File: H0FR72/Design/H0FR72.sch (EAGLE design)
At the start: 49 parts, among them P1 HEXABIT_17.32_NO_P6_P7_P12, Q1 MMBT3904LT1, Q2 STD36P4LLF6, U1 STM32G0B1CEU6N, U2 TSV772IYDT, U3 PMD3001D,115, X1 XTALL_CSTCE8M00G52

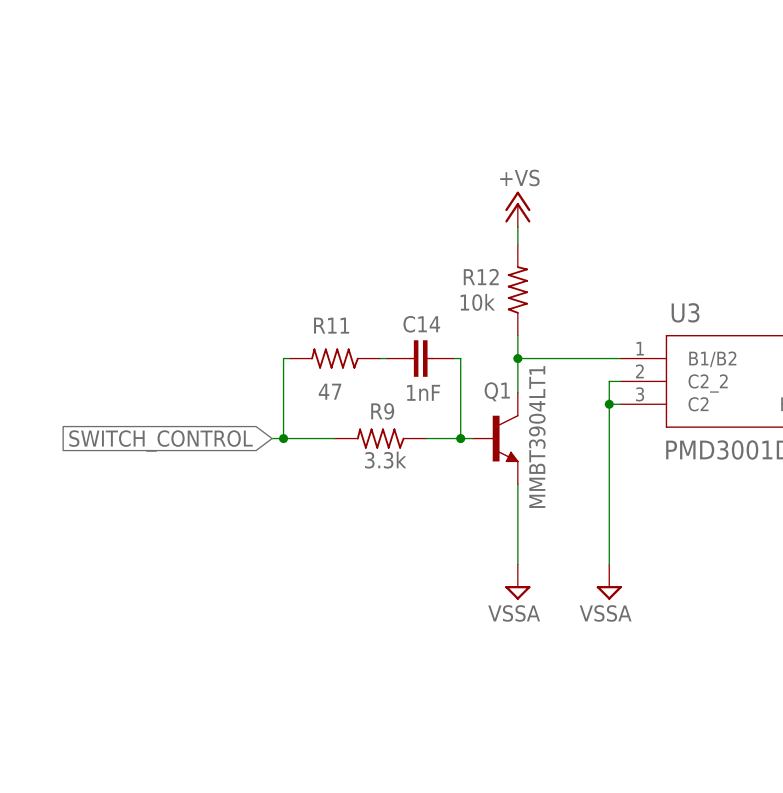
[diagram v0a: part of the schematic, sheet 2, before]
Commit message: Schematic modification
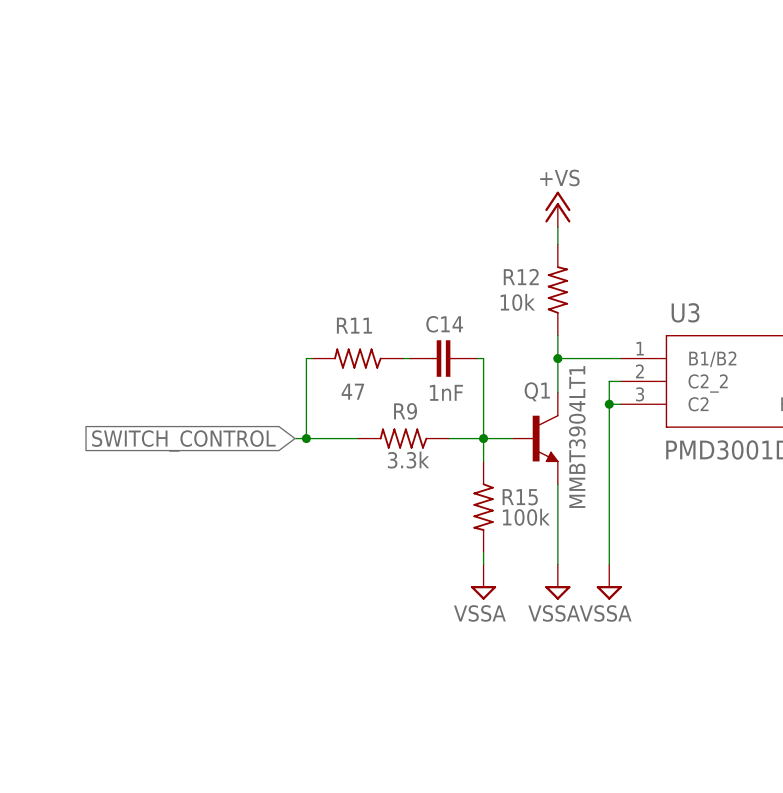
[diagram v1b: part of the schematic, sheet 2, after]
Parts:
- added R15: 100k, HEXABITZ_RCLS:R-0402
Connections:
- net N$14: now also R15.1
- net VSSA: now also R15.2
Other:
- moved on the sheet: C14, Q1, R11, R12, R9
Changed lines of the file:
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@@
 <part name="SUPPLY18" library="supply2" deviceset="VDD" device=""/>
 <part name="SUPPLY19" library="HEXABITZ_CONNECTION_PARTS" library_urn="urn:adsk.eagle:library:20064553" deviceset="VSSA" device=""/>
+<part name="R15" library="HEXABITZ_RCLS" library_urn="urn:adsk.eagle:library:20064561" deviceset="R-0402" device="" package3d_urn="urn:adsk.eagle:package:19666455/3" value="100k">
+<attribute name="MFN" value="Yageo"/>
+<attribute name="MPN" value="RC0603JR-07680KL"/>
+<attribute name="OCTOPART_URL" value="https://octopart.com/rc0603jr-07680kl-yageo-40953169?r=sp"/>
+<attribute name="RESISTANCE" value="680K Ohm"/>
+<attribute name="TOLERANCE" value="5%"/>
+</part>
+<part name="SUPPLY21" library="HEXABITZ_CONNECTION_PARTS" library_urn="urn:adsk.eagle:library:20064553" deviceset="VSSA" device=""/>
 </parts>
 <sheets>
@@
 <attribute name="VALUE" x="249.555" y="85.09" size="1.778" layer="96" rot="R180"/>
 </instance>
-<instance part="R12" gate="G$1" x="64.77" y="135.89" smashed="yes" rot="R90">
-<attribute name="NAME" x="62.865" y="138.2014" size="1.778" layer="95" rot="R180"/>
-<attribute name="VALUE" x="62.23" y="135.382" size="1.778" layer="96" rot="R180"/>
+<instance part="R12" gate="G$1" x="69.215" y="135.89" smashed="yes" rot="R90">
+<attribute name="NAME" x="67.31" y="138.2014" size="1.778" layer="95" rot="R180"/>
+<attribute name="VALUE" x="66.675" y="135.382" size="1.778" layer="96" rot="R180"/>
 </instance>
 <instance part="R5" gate="G$1" x="120.65" y="127.635" smashed="yes" rot="R180">
@@
 <attribute name="POWER" x="124.46" y="126.365" size="1.778" layer="96" rot="R180"/>
 </instance>
-<instance part="Q1" gate="G$1" x="62.23" y="119.38" smashed="yes">
-<attribute name="NAME" x="60.96" y="123.825" size="1.778" layer="95"/>
-<attribute name="VALUE" x="66.04" y="127.635" size="1.778" layer="96" rot="R270"/>
+<instance part="Q1" gate="G$1" x="66.675" y="119.38" smashed="yes">
+<attribute name="NAME" x="65.405" y="123.825" size="1.778" layer="95"/>
+<attribute name="VALUE" x="70.485" y="127.635" size="1.778" layer="96" rot="R270"/>
 </instance>
 <instance part="U3" gate="A" x="91.44" y="125.73" smashed="yes">
@@
 <attribute name="VALUE" x="116.84" y="140.843" size="1.778" layer="96"/>
 </instance>
-<instance part="R9" gate="G$1" x="49.53" y="119.38" smashed="yes" rot="R180">
-<attribute name="NAME" x="48.26" y="121.5136" size="1.778" layer="95"/>
-<attribute name="VALUE" x="47.625" y="116.078" size="1.778" layer="96"/>
-</instance>
-<instance part="C14" gate="G$1" x="55.245" y="128.27" smashed="yes" rot="R90">
-<attribute name="NAME" x="56.261" y="132.969" size="1.778" layer="95" rot="R180"/>
-<attribute name="VALUE" x="56.261" y="125.349" size="1.778" layer="96" rot="R180"/>
-</instance>
-<instance part="R11" gate="G$1" x="44.45" y="128.27" smashed="yes" rot="R180">
-<attribute name="NAME" x="41.91" y="131.0386" size="1.778" layer="95"/>
-<attribute name="VALUE" x="42.545" y="123.698" size="1.778" layer="96"/>
+<instance part="R9" gate="G$1" x="52.07" y="119.38" smashed="yes" rot="R180">
+<attribute name="NAME" x="50.8" y="121.5136" size="1.778" layer="95"/>
+<attribute name="VALUE" x="50.165" y="116.078" size="1.778" layer="96"/>
+</instance>
+<instance part="C14" gate="G$1" x="57.785" y="128.27" smashed="yes" rot="R90">
+<attribute name="NAME" x="58.801" y="132.969" size="1.778" layer="95" rot="R180"/>
+<attribute name="VALUE" x="58.801" y="125.349" size="1.778" layer="96" rot="R180"/>
+</instance>
+<instance part="R11" gate="G$1" x="46.99" y="128.27" smashed="yes" rot="R180">
+<attribute name="NAME" x="44.45" y="131.0386" size="1.778" layer="95"/>
+<attribute name="VALUE" x="45.085" y="123.698" size="1.778" layer="96"/>
 </instance>
 <instance part="P+1" gate="1" x="15.875" y="198.755" smashed="yes">
@@
 <attribute name="VALUE" x="161.925" y="187.96" size="1.778" layer="96" rot="R180"/>
 </instance>
-<instance part="SUPPLY12" gate="G$1" x="64.77" y="102.87" smashed="yes">
-<attribute name="VALUE" x="61.468" y="99.06" size="1.778" layer="96"/>
+<instance part="SUPPLY12" gate="G$1" x="69.215" y="102.87" smashed="yes">
+<attribute name="VALUE" x="65.913" y="99.06" size="1.778" layer="96"/>
 </instance>
 <instance part="C15" gate="G$1" x="167.64" y="179.705" smashed="yes" rot="R270">
@@
 <attribute name="VALUE" x="110.49" y="157.48" size="1.778" layer="96" rot="R180"/>
 </instance>
-<instance part="P+4" gate="1" x="64.77" y="145.415" smashed="yes">
-<attribute name="VALUE" x="67.31" y="149.225" size="1.778" layer="96" rot="R180"/>
+<instance part="P+4" gate="1" x="69.215" y="145.415" smashed="yes">
+<attribute name="VALUE" x="71.755" y="149.225" size="1.778" layer="96" rot="R180"/>
 </instance>
 <instance part="SUPPLY19" gate="G$1" x="167.64" y="162.56" smashed="yes">
 <attribute name="VALUE" x="164.338" y="158.75" size="1.778" layer="96"/>
 </instance>
+<instance part="R15" gate="G$1" x="60.96" y="111.76" smashed="yes" rot="R270">
+<attribute name="NAME" x="62.865" y="111.9886" size="1.778" layer="95"/>
+<attribute name="VALUE" x="62.865" y="109.728" size="1.778" layer="96"/>
+</instance>
+<instance part="SUPPLY21" gate="G$1" x="60.96" y="102.87" smashed="yes">
+<attribute name="VALUE" x="57.658" y="99.06" size="1.778" layer="96"/>
+</instance>
 </instances>
 <busses>
@@
 <segment>
 <pinref part="R9" gate="G$1" pin="1"/>
-<wire x1="54.61" y1="119.38" x2="58.42" y2="119.38" width="0.1524" layer="91"/>
+<wire x1="57.15" y1="119.38" x2="60.96" y2="119.38" width="0.1524" layer="91"/>
 <pinref part="Q1" gate="G$1" pin="B"/>
-<wire x1="59.69" y1="119.38" x2="58.42" y2="119.38" width="0.1524" layer="91"/>
+<wire x1="64.135" y1="119.38" x2="60.96" y2="119.38" width="0.1524" layer="91"/>
 <pinref part="C14" gate="G$1" pin="2"/>
-<wire x1="57.785" y1="128.27" x2="58.42" y2="128.27" width="0.1524" layer="91"/>
-<wire x1="58.42" y1="128.27" x2="58.42" y2="119.38" width="0.1524" layer="91"/>
-<junction x="58.42" y="119.38"/>
+<wire x1="60.325" y1="128.27" x2="60.96" y2="128.27" width="0.1524" layer="91"/>
+<wire x1="60.96" y1="128.27" x2="60.96" y2="119.38" width="0.1524" layer="91"/>
+<junction x="60.96" y="119.38"/>
+<pinref part="R15" gate="G$1" pin="1"/>
+<wire x1="60.96" y1="116.84" x2="60.96" y2="119.38" width="0.1524" layer="91"/>
 </segment>
 </net>
@@
 <pinref part="R11" gate="G$1" pin="1"/>
 <pinref part="C14" gate="G$1" pin="1"/>
-<wire x1="49.53" y1="128.27" x2="50.165" y2="128.27" width="0.1524" layer="91"/>
+<wire x1="52.07" y1="128.27" x2="52.705" y2="128.27" width="0.1524" layer="91"/>
 </segment>
 </net>
@@
 <segment>
 <pinref part="R11" gate="G$1" pin="2"/>
-<wire x1="39.37" y1="128.27" x2="38.735" y2="128.27" width="0.1524" layer="91"/>
-<wire x1="38.735" y1="128.27" x2="38.735" y2="119.38" width="0.1524" layer="91"/>
-<label x="37.465" y="119.38" size="1.778" layer="95" rot="MR0" xref="yes"/>
+<wire x1="41.91" y1="128.27" x2="41.275" y2="128.27" width="0.1524" layer="91"/>
+<wire x1="41.275" y1="128.27" x2="41.275" y2="119.38" width="0.1524" layer="91"/>
+<label x="40.005" y="119.38" size="1.778" layer="95" rot="MR0" xref="yes"/>
 <pinref part="R9" gate="G$1" pin="2"/>
-<wire x1="38.735" y1="119.38" x2="37.465" y2="119.38" width="0.1524" layer="91"/>
-<wire x1="44.45" y1="119.38" x2="38.735" y2="119.38" width="0.1524" layer="91"/>
-<junction x="38.735" y="119.38"/>
+<wire x1="41.275" y1="119.38" x2="40.005" y2="119.38" width="0.1524" layer="91"/>
+<wire x1="46.99" y1="119.38" x2="41.275" y2="119.38" width="0.1524" layer="91"/>
+<junction x="41.275" y="119.38"/>
 </segment>
 </net>
@@
 <segment>
 <pinref part="R12" gate="G$1" pin="2"/>
-<wire x1="64.77" y1="140.97" x2="64.77" y2="142.875" width="0.1524" layer="91"/>
+<wire x1="69.215" y1="140.97" x2="69.215" y2="142.875" width="0.1524" layer="91"/>
 <pinref part="P+4" gate="1" pin="+VS"/>
 </segment>
@@
 <pinref part="Q1" gate="G$1" pin="E"/>
 <pinref part="SUPPLY12" gate="G$1" pin="VSSA"/>
-<wire x1="64.77" y1="114.3" x2="64.77" y2="105.41" width="0.1524" layer="91"/>
+<wire x1="69.215" y1="114.3" x2="69.215" y2="105.41" width="0.1524" layer="91"/>
 </segment>
 <segment>
@@
 <wire x1="167.64" y1="165.1" x2="167.64" y2="167.005" width="0.1524" layer="91"/>
 </segment>
+<segment>
+<pinref part="R15" gate="G$1" pin="2"/>
+<pinref part="SUPPLY21" gate="G$1" pin="VSSA"/>
+<wire x1="60.96" y1="106.68" x2="60.96" y2="105.41" width="0.1524" layer="91"/>
+</segment>
 </net>
 <net name="N$16" class="0">
@@
 <pinref part="Q1" gate="G$1" pin="C"/>
 <pinref part="R12" gate="G$1" pin="1"/>
-<wire x1="64.77" y1="130.81" x2="64.77" y2="128.27" width="0.1524" layer="91"/>
+<wire x1="69.215" y1="130.81" x2="69.215" y2="128.27" width="0.1524" layer="91"/>
 <pinref part="U3" gate="A" pin="B1/B2"/>
-<wire x1="64.77" y1="128.27" x2="64.77" y2="124.46" width="0.1524" layer="91"/>
-<wire x1="76.2" y1="128.27" x2="64.77" y2="128.27" width="0.1524" layer="91"/>
-<junction x="64.77" y="128.27"/>
+<wire x1="69.215" y1="128.27" x2="69.215" y2="124.46" width="0.1524" layer="91"/>
+<wire x1="76.2" y1="128.27" x2="69.215" y2="128.27" width="0.1524" layer="91"/>
+<junction x="69.215" y="128.27"/>
 </segment>
 </net>
